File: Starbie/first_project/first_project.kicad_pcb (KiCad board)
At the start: 2 copper layers, 92.5 x 71.6 mm, 7 parts, among them J1 Conn_01x04_Pin, J2 Conn_01x08_Pin, SW1 SW_Push, SW2 SW_Push, U1 DHT11, U2 XIAO-ESP32-C3-SMD

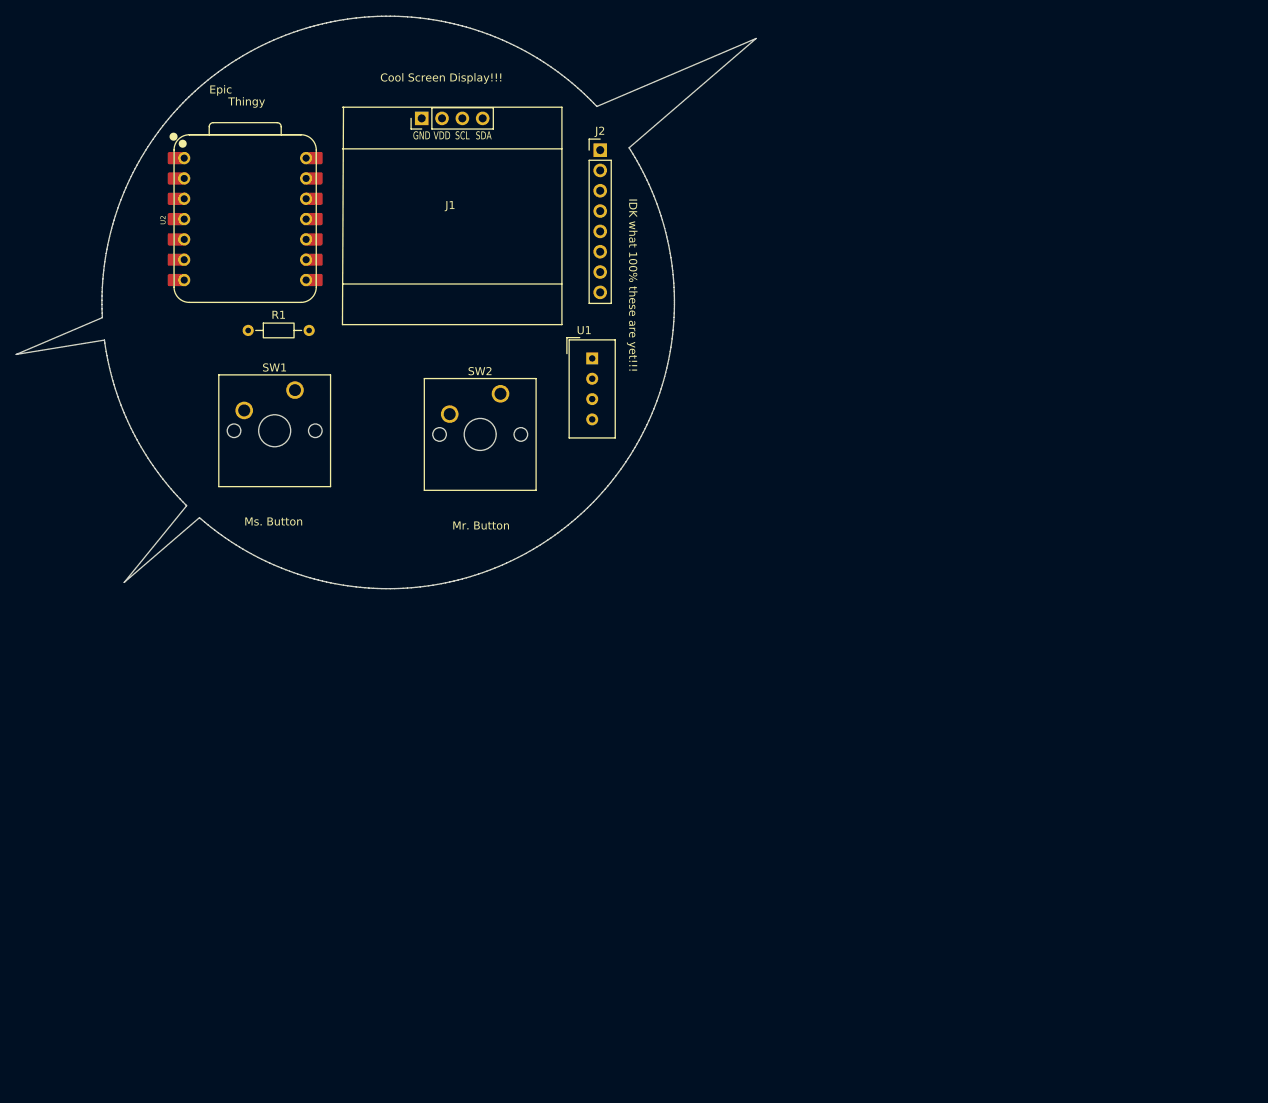
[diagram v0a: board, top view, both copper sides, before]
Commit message: ChromeOS Migration
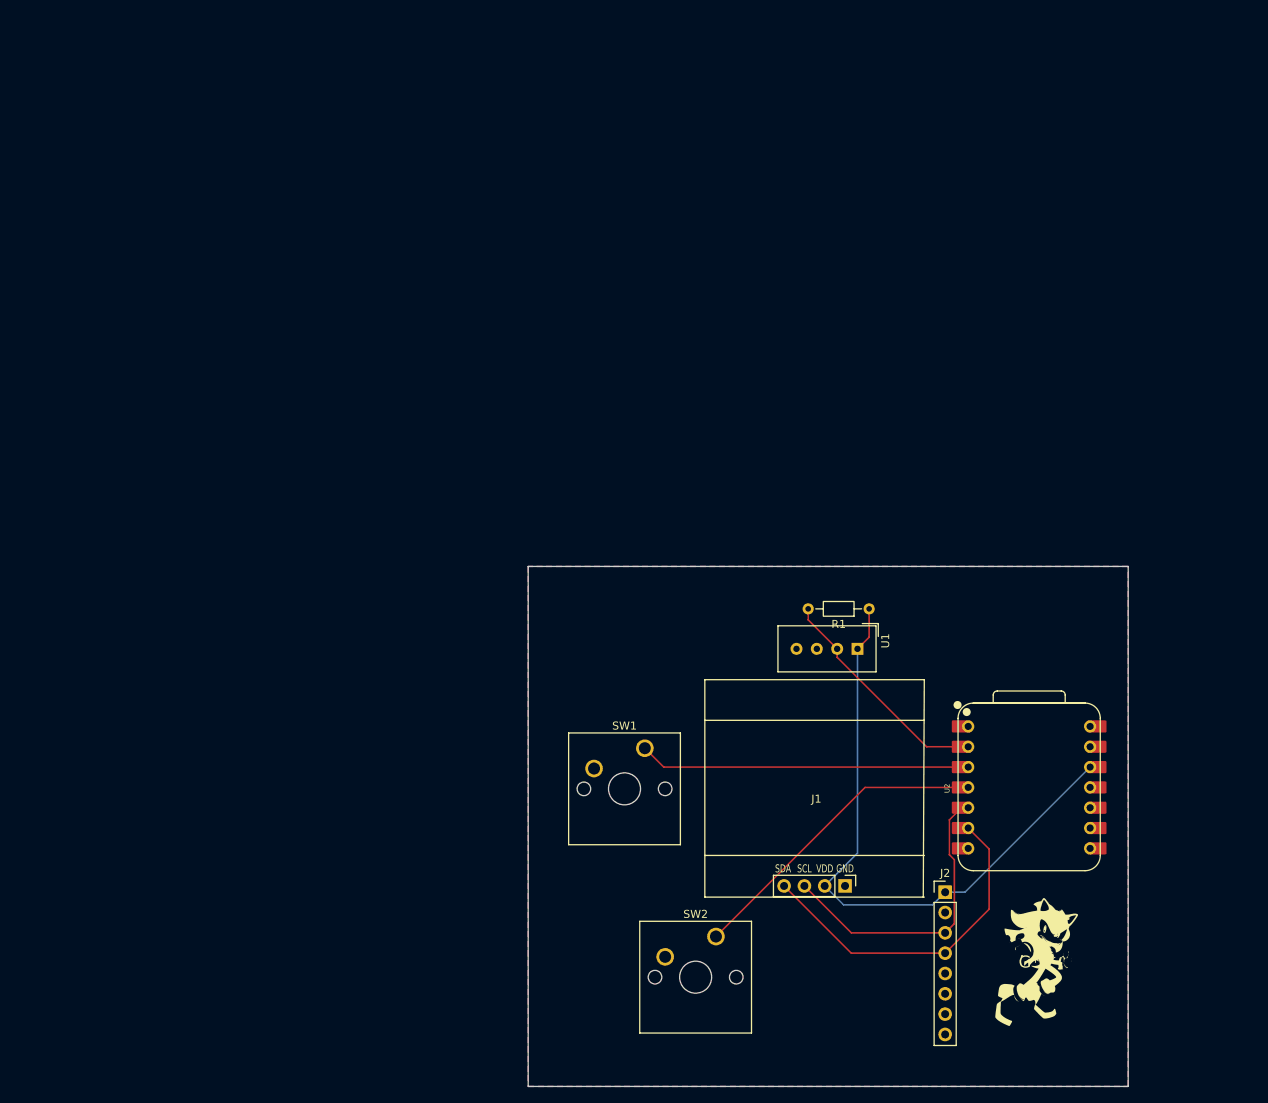
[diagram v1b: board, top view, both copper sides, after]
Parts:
- added G***: LOGO, LOGO, F.Cu at (213.6, 149.4)
- moved U2 121.0 mm to (212.6, 127.6)
- moved J1 106.1 mm to (185.8, 139.9), turned to 180 degrees
- moved J2 102.3 mm to (202.1, 140.7)
- moved R1 85.1 mm to (192.6, 105.3), turned to 180 degrees
- moved SW2 73.0 mm to (173.5, 146.3)
- moved SW1 62.6 mm to (164.6, 122.7)
- moved U1 49.2 mm to (191.2, 110.3), turned to -90 degrees
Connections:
- SW2 pad 1: /GPI03 -> /GPIO3
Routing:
- net +3.3V: track 0.00 -> 78.2 mm
- net /SDA: track 0.00 -> 42.6 mm
- net /GPIO2: track 0.00 -> 40.6 mm
- net /GPIO3: track 0.00 -> 39.3 mm
- net /SCL: track 0.00 -> 37.9 mm
- net /DHT11 DATA: track 0.00 -> 28.6 mm
- added copper zone on B.Cu, net GND
- added copper zone on F.Cu, net GND
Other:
- board size 92.5 x 71.6 mm -> 75 x 65 mm
- board text removed: "Cool Screen Display!!!"
- board text removed: "Epic"
- board text removed: "IDK what 100% these are yet!!!"
- board text removed: "Mr. Button"
- board text removed: "Ms. Button"
- board text removed: "Thingy"

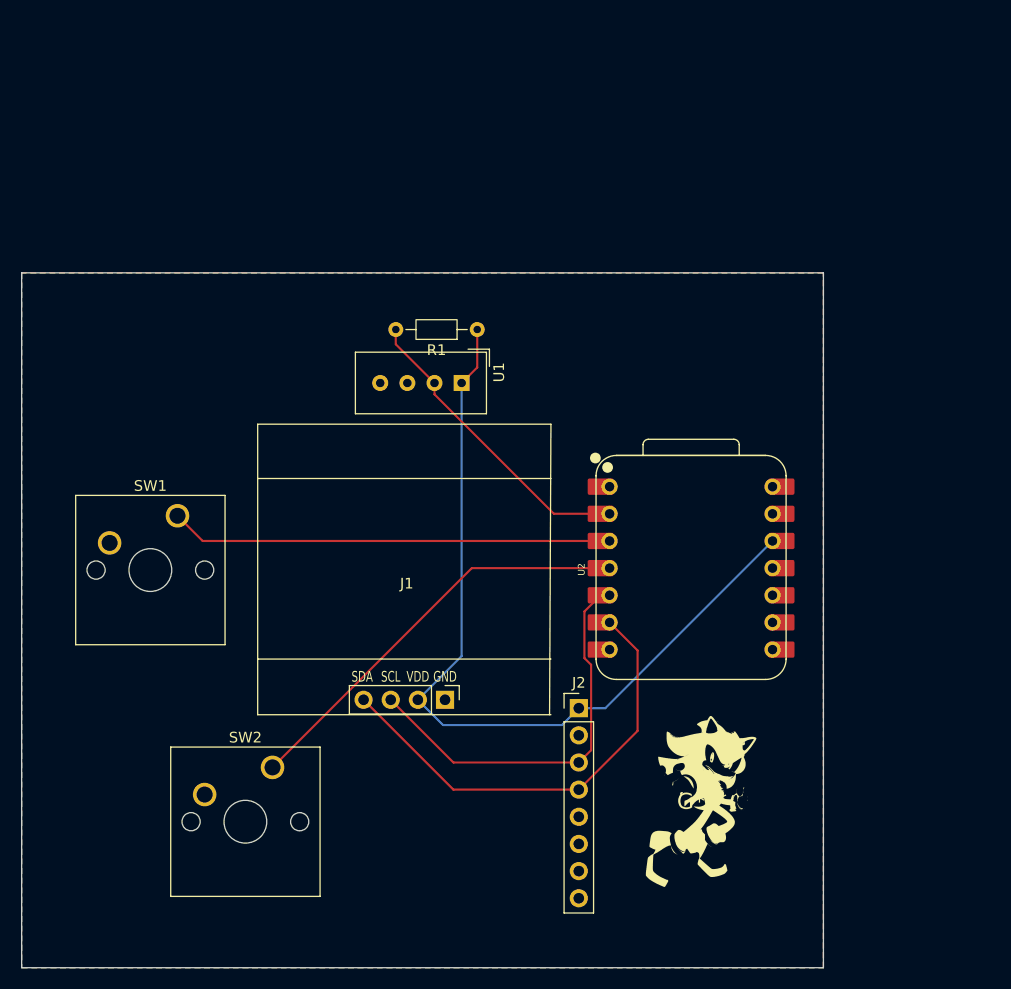
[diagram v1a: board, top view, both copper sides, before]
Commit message: Update first_project.kicad_pcb
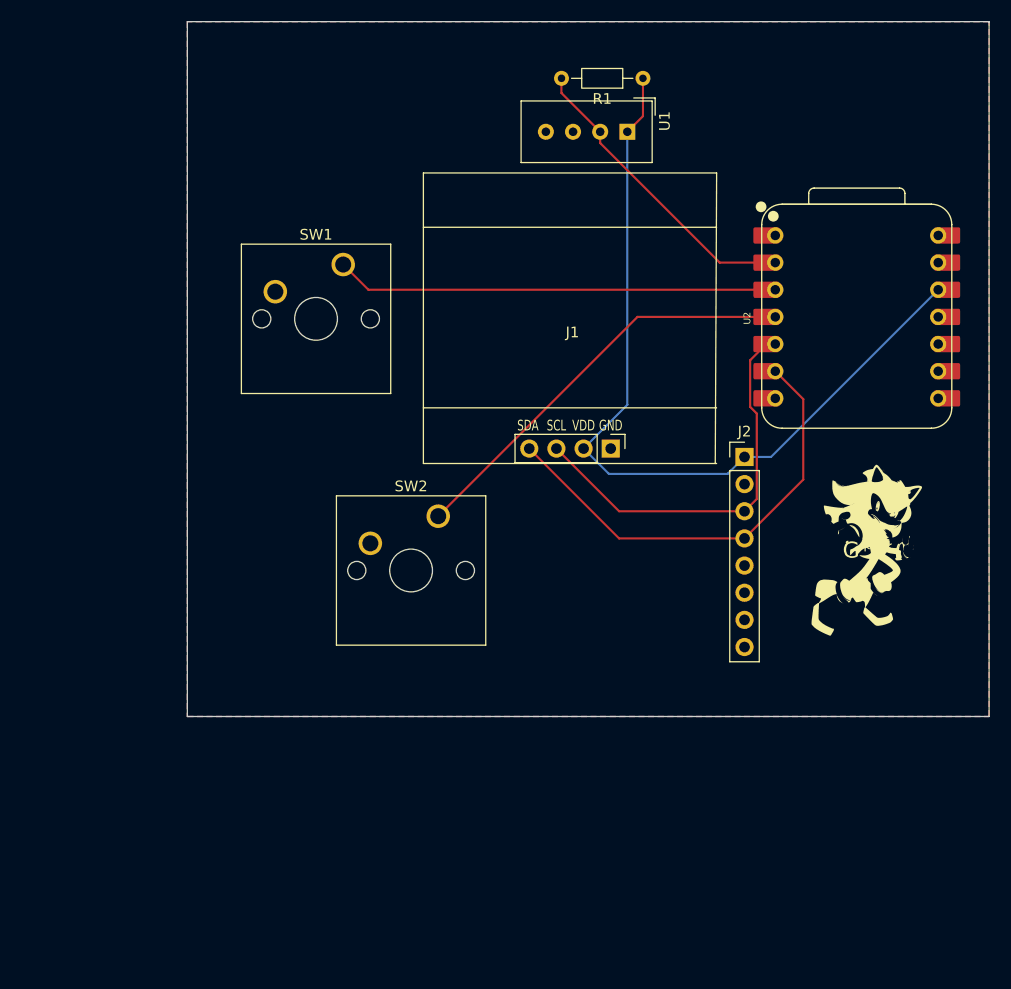
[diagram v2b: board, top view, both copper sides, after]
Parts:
- moved G*** 28.2 mm to (229.1, 125.9)
- moved SW2 28.2 mm to (189.0, 122.8)
- moved J1 28.2 mm to (201.3, 116.4)
- moved R1 28.2 mm to (208.1, 81.8)
- moved SW1 28.2 mm to (180.1, 99.2)
- moved U1 28.2 mm to (206.7, 86.8)
- moved U2 28.2 mm to (228.1, 104.1)
- moved J2 28.2 mm to (217.6, 117.2)
